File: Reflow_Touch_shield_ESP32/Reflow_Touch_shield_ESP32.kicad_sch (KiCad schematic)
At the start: 38 parts, among them IC1 MAX6675, J1 Conn_01x14, J2 Jack-DC, J3 , J4 Conn_01x04_MountingPin, Q1 FDN340P, SW1 SW_Push, U1 LM358, U2 AMS1117-3.3, U3 ESP32-WROOM-32D, U4 AMS1117-5.0, U5 CH340C

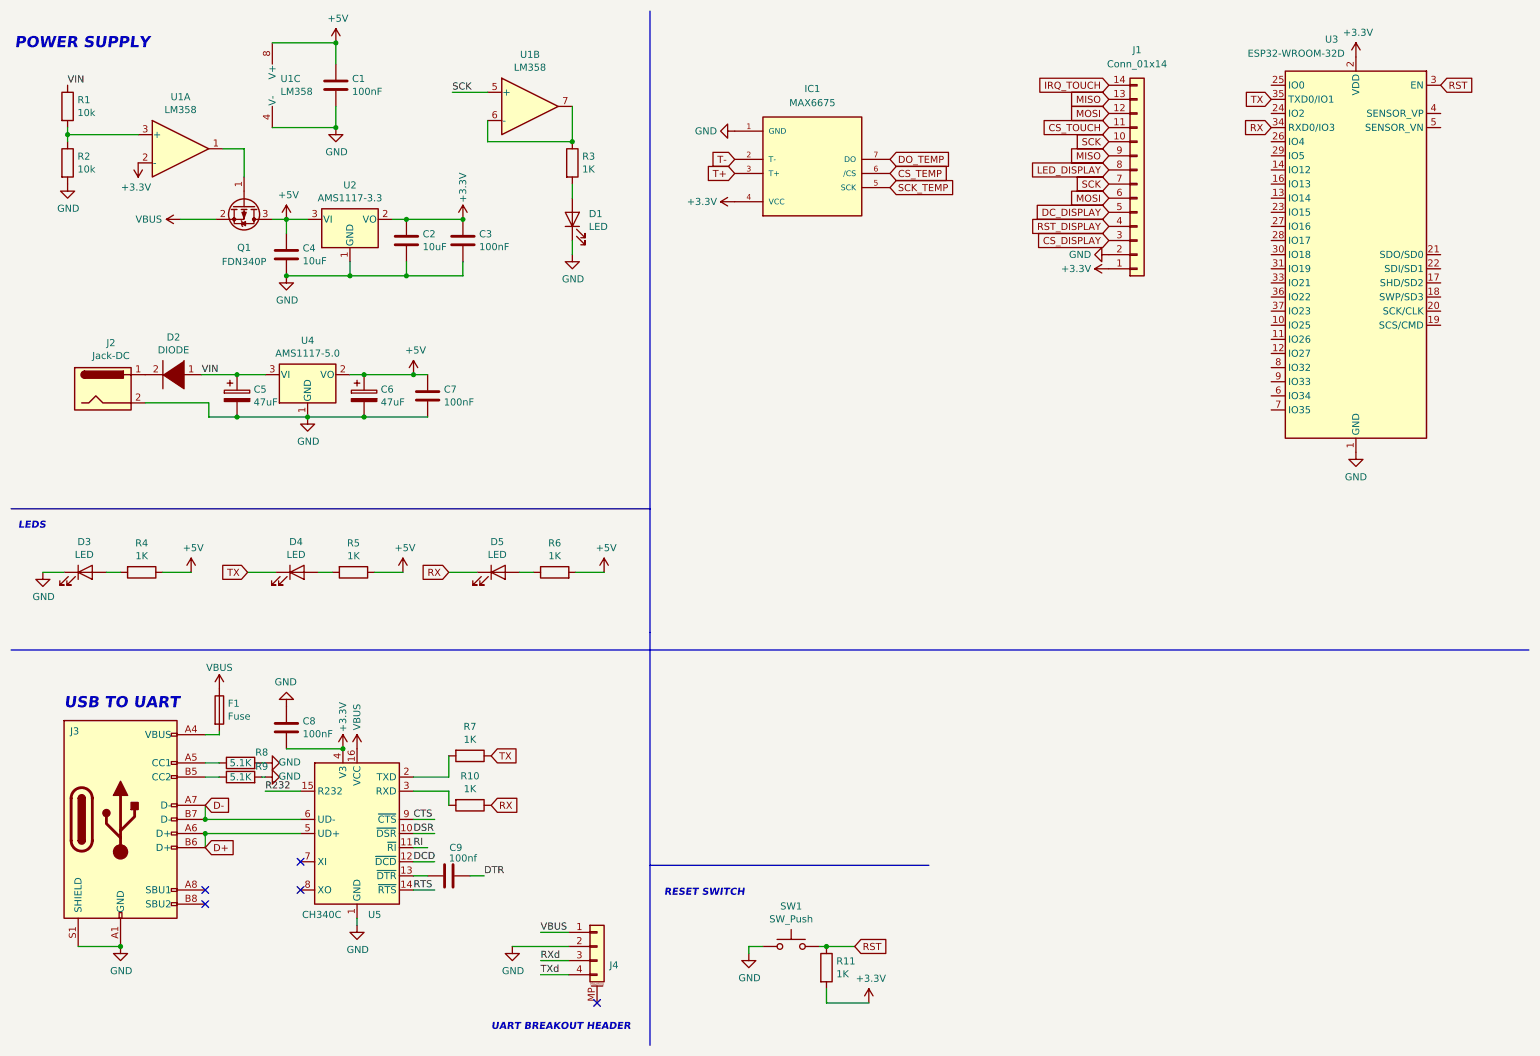
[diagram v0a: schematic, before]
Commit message: update
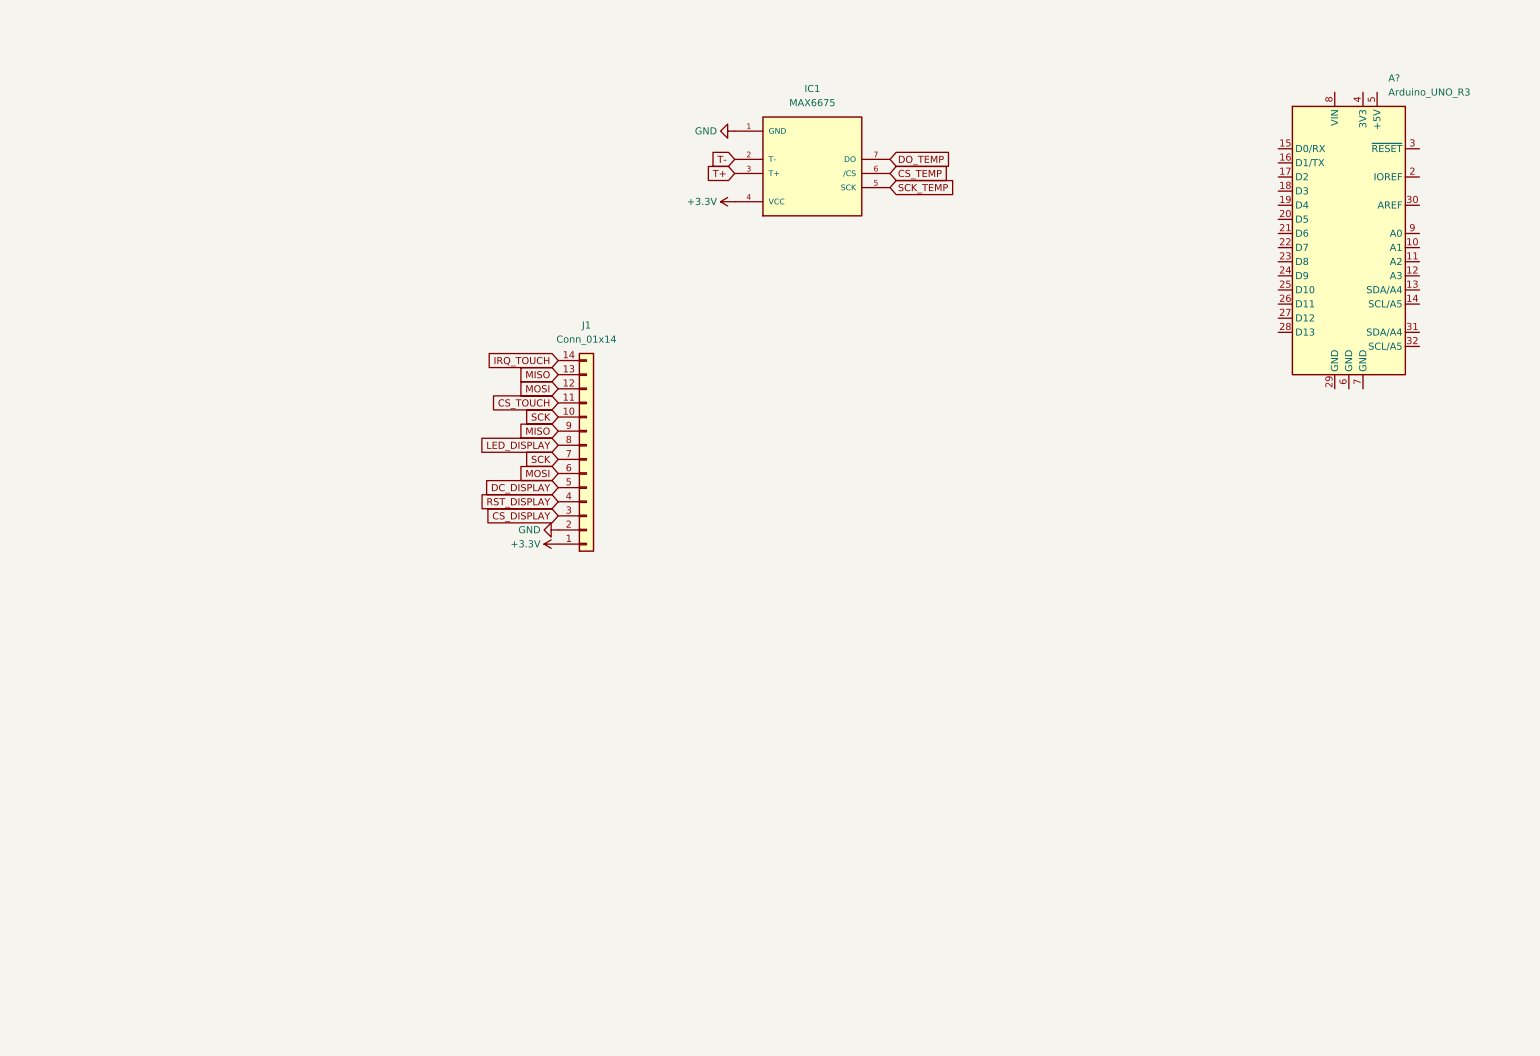
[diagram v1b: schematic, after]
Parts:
- removed C1, C3, C7, C8: 100nF, Capacitor_SMD:C_0603_1608Metric_Pad1.08x0.95mm_HandSolder, symbol stormduino-Rev2-rescue:C-Device
- removed C2, C4: 10uF, Capacitor_SMD:C_0603_1608Metric_Pad1.08x0.95mm_HandSolder, symbol stormduino-Rev2-rescue:C-Device
- removed C5, C6: 47uF, Capacitor_SMD:CP_Elec_4x3, symbol stormduino-Rev2-rescue:CP-Device
- removed C9: 100nf, Capacitor_SMD:C_0603_1608Metric_Pad1.08x0.95mm_HandSolder, symbol stormduino-Rev2-rescue:C-Device
- removed D1, D3, D4, D5: LED, LED_SMD:LED_0603_1608Metric_Pad1.05x0.95mm_HandSolder, symbol stormduino-Rev2-rescue:LED-Device
- removed D2: DIODE, Diode_SMD:D_SOD-128, symbol stormduino-Rev2-rescue:DIODE-pspice
- removed F1: Fuse, symbol stormduino-Rev2-rescue:Fuse-Device
- removed J2: Jack-DC, Connector_BarrelJack:BarrelJack_Horizontal, symbol stormduino-Rev2-rescue:Jack-DC-Connector
- removed J3: (no value), kien242:USB-C-16pin-hight-v2, symbol Connector:USB_C_Receptacle_USB2.0
- removed J4: Conn_01x04_MountingPin, symbol stormduino-Rev2-rescue:Conn_01x04_MountingPin-Connector_Generic_MountingPin
- removed Q1: FDN340P, Package_TO_SOT_SMD:SOT-23_Handsoldering, symbol Transistor_FET:FDN340P
- removed R1, R2: 10k, Resistor_SMD:R_0603_1608Metric_Pad0.98x0.95mm_HandSolder, symbol stormduino-Rev2-rescue:R-Device
- removed R10, R11, R3, R4, R5, R6, R7: 1K, Resistor_SMD:R_0603_1608Metric_Pad0.98x0.95mm_HandSolder, symbol stormduino-Rev2-rescue:R-Device
- removed R8, R9: 5.1K, Resistor_SMD:R_0603_1608Metric_Pad0.98x0.95mm_HandSolder, symbol stormduino-Rev2-rescue:R-Device
- removed SW1: SW_Push, symbol stormduino-Rev2-rescue:SW_Push-Switch
- removed U1: LM358, Package_SO:SOP-8_3.9x4.9mm_P1.27mm, symbol stormduino-Rev2-rescue:LM358-Amplifier_Operational
- removed U2: AMS1117-3.3, Package_TO_SOT_SMD:SOT-223-3_TabPin2, symbol stormduino-Rev2-rescue:AMS1117-3.3-Regulator_Linear
- removed U3: ESP32-WROOM-32D, RF_Module:ESP32-WROOM-32, symbol RF_Module:ESP32-WROOM-32D
- removed U4: AMS1117-5.0, Package_TO_SOT_SMD:SOT-223-3_TabPin2, symbol stormduino-Rev2-rescue:AMS1117-5.0-Regulator_Linear
- removed U5: CH340C, Package_SO:SOIC-16_3.9x9.9mm_P1.27mm, symbol stormduino-Rev2-rescue:CH340G-Interface_USB
- added A?: Arduino_UNO_R3, Module:Arduino_UNO_R3, symbol MCU_Module:Arduino_UNO_R3
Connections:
- no-connect marks 5 -> 0
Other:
- note removed: "LEDS"
- note removed: "POWER SUPPLY"
- note removed: "RESET SWITCH"
- note removed: "UART BREAKOUT HEADER"
- note removed: "USB TO UART"
- moved on the sheet: J1
